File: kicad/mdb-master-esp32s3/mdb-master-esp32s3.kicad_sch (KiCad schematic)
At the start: 36 parts, among them J2 MDB_Connector, J3 Conn_02x09_Odd_Even, P1 USB_C_Plug_USB2.0, SW1 SW_Push, U1 ESP32-S3, U2 W25Q32JVSS, U4 LM317_SOT-223, U5 PC817, U6 PC817, Y1 Crystal

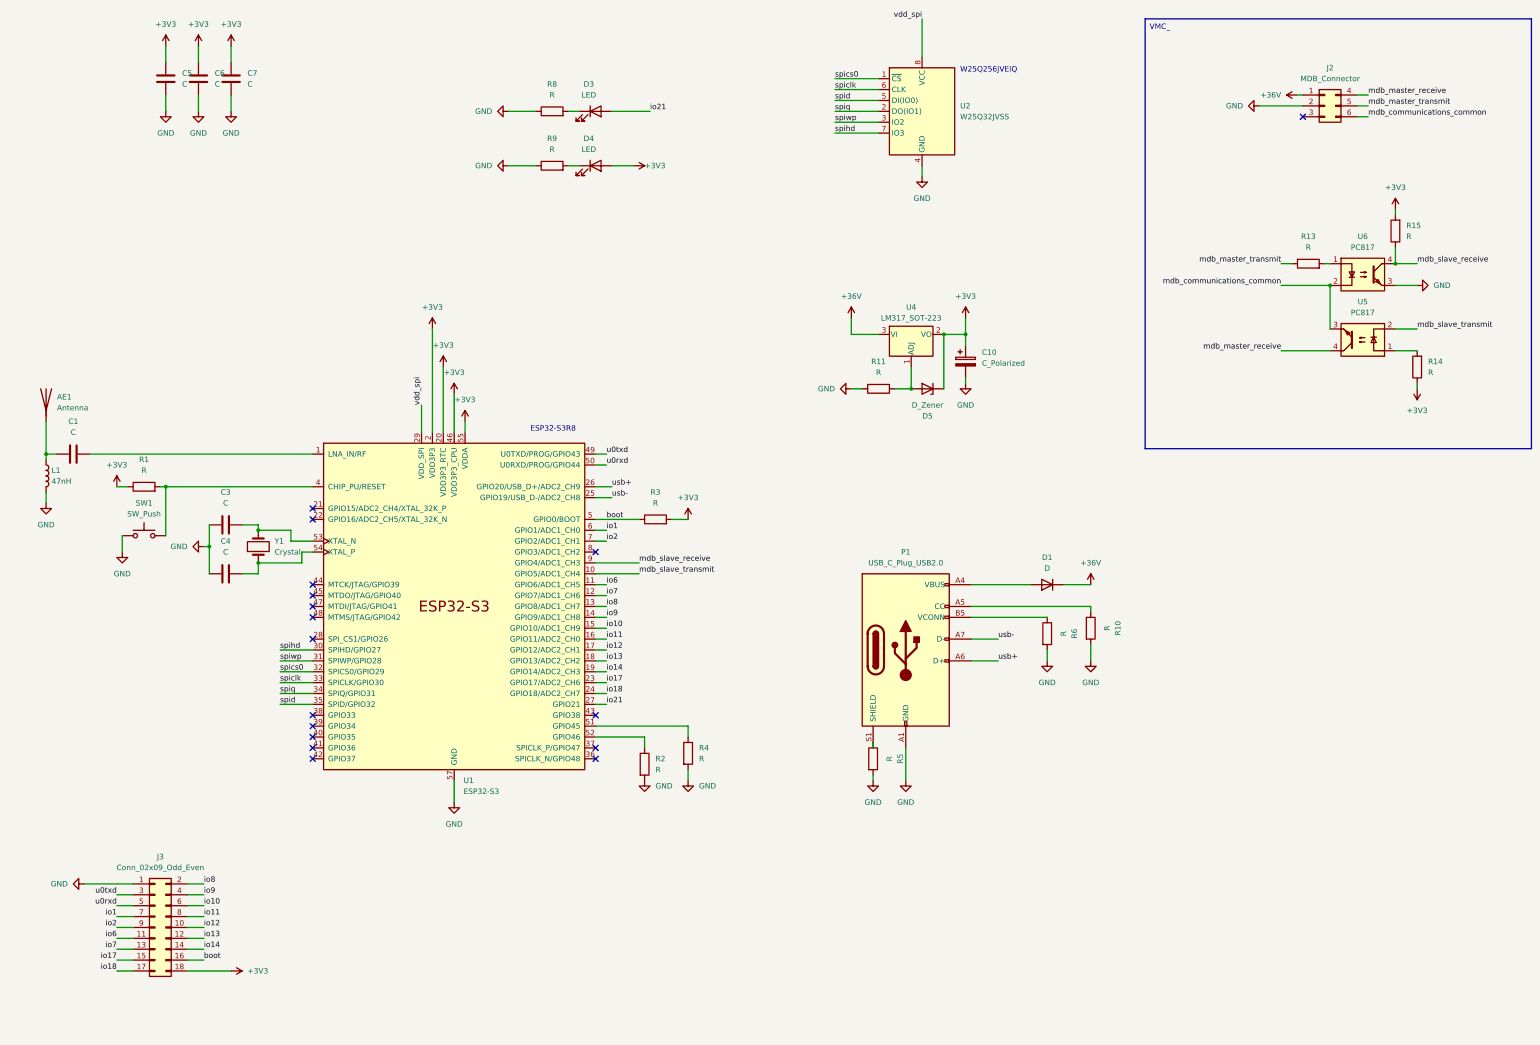
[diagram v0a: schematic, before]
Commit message: Refacting
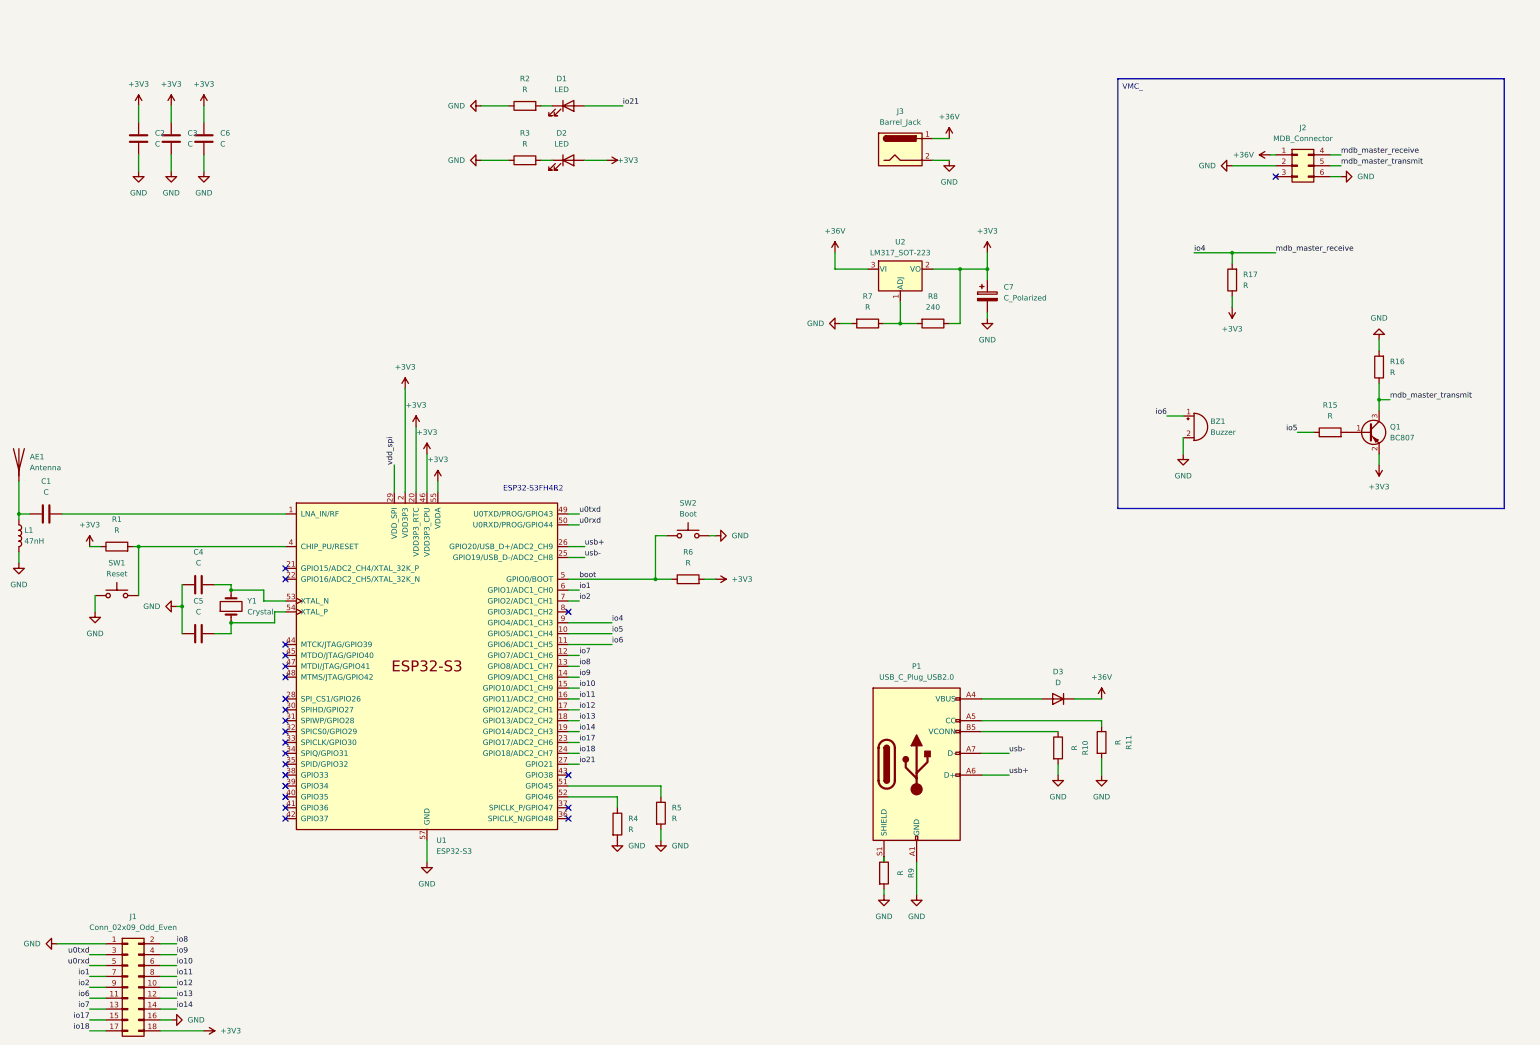
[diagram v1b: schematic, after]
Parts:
- removed C10: C_Polarized, Capacitor_Tantalum_SMD:CP_EIA-3216-18_Kemet-A, symbol Device:C_Polarized
- removed C7: C, Capacitor_SMD:C_0603_1608Metric, symbol Device:C
- removed D1: D, Diode_SMD:D_SOD-123, symbol Device:D
- removed D3, D4: LED, LED_SMD:LED_0603_1608Metric, symbol Device:LED
- removed D5: D_Zener, Diode_SMD:D_MiniMELF, symbol Device:D_Zener
- removed J3: Conn_02x09_Odd_Even, Connector_PinHeader_2.54mm:PinHeader_2x09_P2.54mm_Vertical, symbol Connector_Generic:Conn_02x09_Odd_Even
- removed R13, R14: R, Resistor_SMD:R_0805_2012Metric, symbol Device:R
- removed U2: W25Q32JVSS, Package_SON:WSON-8-1EP_8x6mm_P1.27mm_EP3.4x4.3mm, symbol Memory_Flash:W25Q32JVSS
- removed U4: LM317_SOT-223, Package_TO_SOT_SMD:SOT-223-3_TabPin2, symbol Regulator_Linear:LM317_SOT-223
- removed U5, U6: PC817, Package_DIP:DIP-4_W7.62mm, symbol Isolator:PC817
- added BZ1: Buzzer, Buzzer_Beeper:Buzzer_12x9.5RM7.6, symbol Device:Buzzer
- added C2: C, Capacitor_SMD:C_0603_1608Metric, symbol Device:C
- added C7: C_Polarized, Capacitor_Tantalum_SMD:CP_EIA-3216-18_Kemet-A, symbol Device:C_Polarized
- added D1, D2: LED, LED_SMD:LED_0603_1608Metric, symbol Device:LED
- added D3: D, Diode_SMD:D_SOD-123, symbol Device:D
- added J1: Conn_02x09_Odd_Even, Connector_PinHeader_2.54mm:PinHeader_2x09_P2.54mm_Vertical, symbol Connector_Generic:Conn_02x09_Odd_Even
- added J3: Barrel_Jack, Connector_BarrelJack:BarrelJack_Horizontal, symbol Connector:Barrel_Jack
- added Q1: BC807, Package_TO_SOT_SMD:SOT-23, symbol Transistor_BJT:BC807
- added R16, R17, R7: R, Resistor_SMD:R_0603_1608Metric, symbol Device:R
- added SW2: Boot, Button_Switch_SMD:SW_Tactile_SPST_NO_Straight_CK_PTS636Sx25SMTRLFS, symbol Switch:SW_Push
- added U2: LM317_SOT-223, Package_TO_SOT_SMD:SOT-223-3_TabPin2, symbol Regulator_Linear:LM317_SOT-223
- R11, R15: footprint Resistor_SMD:R_0805_2012Metric -> Resistor_SMD:R_0603_1608Metric
- R8: value R -> 240
- SW1: value SW_Push -> Reset
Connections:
- net mdb_communications_common is gone; now on net GND: J2.6 (Pin_6)
- net mdb_slave_transmit is gone; now on net io5: U1.10 (GPIO5/ADC1_CH4)
- net +36V: now also D3.1 (K), J3.1, U2.3 (VI)
- net +3V3: now also C3.2, R6.2, R8.1, C2.2, C7.1, D2.2 (A), J1.18 (Pin_18), Q1.2 (E), R17.1, U2.2 (VO); no longer C5.2, R15.2, R3.2
- net GND: now also R2.1, R3.1, R9.2, BZ1.2 (-), C2.1, C7.2, J1.1 (Pin_1), J1.16 (Pin_16), J3.2, R16.2, R7.2, SW2.2; no longer R2.2, R6.2, R8.1, R9.1
- net boot: now also R6.1, SW2.1; no longer R3.1
- net io1: now also J1.7 (Pin_7)
- net io10: now also J1.6 (Pin_6)
- net io11: now also J1.8 (Pin_8)
- net io12: now also J1.10 (Pin_10)
- net io13: now also J1.12 (Pin_12)
- net io14: now also J1.14 (Pin_14)
- net io17: now also J1.15 (Pin_15)
- net io18: now also J1.17 (Pin_17)
- net io2: now also J1.9 (Pin_9)
- net io21: now also D1.2 (A)
- net io6: now also BZ1.1 (+), J1.11 (Pin_11)
- net io7: now also J1.13 (Pin_13)
- net io8: now also J1.2 (Pin_2)
- net io9: now also J1.4 (Pin_4)
- net mdb_master_transmit: now also Q1.3 (C), R16.1
- net u0rxd: now also J1.5 (Pin_5)
- net u0txd: now also J1.3 (Pin_3)
- net at U1.54 (XTAL_P), Y1.1: now also C5.2; no longer C4.2
- net at R8.2: now also R7.1, U2.1 (ADJ)
- net at R11.1: now also P1.A5 (CC)
- net at U1.51 (GPIO45): now also R5.1; no longer R4.1
- net at U1.53 (XTAL_N), Y1.2: now also C4.2; no longer C3.2
- net at U1.52 (GPIO46): now also R4.1; no longer R2.1
- net at P1.A4 (VBUS), P1.A9 (VBUS), P1.B4 (VBUS)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: now also D3.2 (A)
- net at R10.1: now also P1.B5 (VCONN); no longer P1.A5 (CC)
- net at P1.S1 (SHIELD): now also R9.1; no longer R5.1
- net mdb_master_receive renamed io4
- net io4: now also U1.9 (GPIO4/ADC1_CH3), R17.2
- net mdb_slave_receive renamed io5
- net io5: no longer U1.9 (GPIO4/ADC1_CH3)
- net spiclk: no longer names the net of U1.33 (SPICLK/GPIO30)
- net spics0: no longer names the net of U1.32 (SPICS0/GPIO29)
- net spid: no longer names the net of U1.35 (SPID/GPIO32)
- net spihd: no longer names the net of U1.30 (SPIHD/GPIO27)
- net spiq: no longer names the net of U1.34 (SPIQ/GPIO31)
- net spiwp: no longer names the net of U1.31 (SPIWP/GPIO28)
- new net: Q1.1 (B), R15.2
- new net: D2.1 (K), R3.2
- new net: D1.1 (K), R2.2
- no-connect marks 17 -> 23
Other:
- note added: "ESP32-S3FH4R2"
- note removed: "ESP32-S3R8"
- note removed: "W25Q256JVEIQ"
